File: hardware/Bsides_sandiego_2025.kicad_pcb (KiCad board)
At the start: 2 copper layers, 49.9 x 71.1 mm, 33 parts, among them J1 Conn_02x03_Odd_Even, J2 OLED, SW1 RESET, SW2 SW_SPDT, U1 CH32V003FxPx

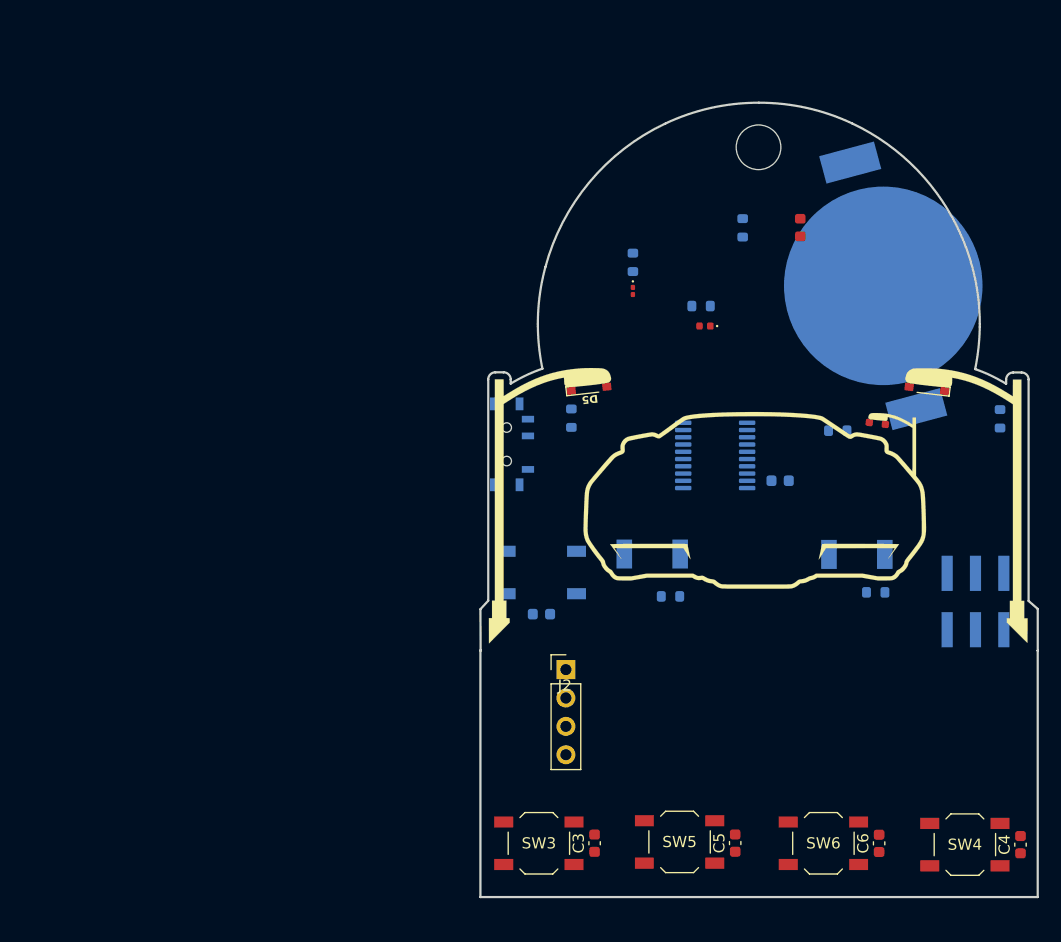
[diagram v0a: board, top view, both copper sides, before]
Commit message: feat(Hw):Update_Route
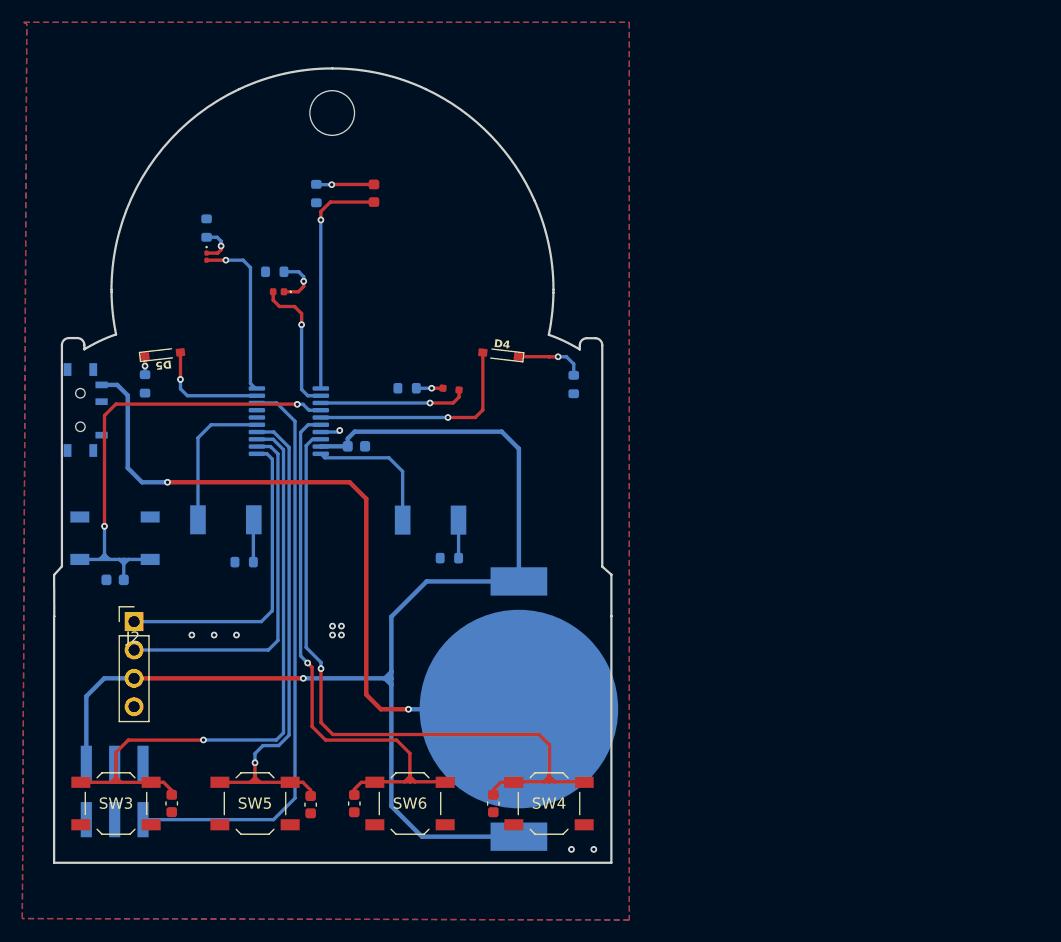
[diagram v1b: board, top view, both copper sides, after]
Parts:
- moved J1 78.9 mm to (67.1, 111.0)
- moved BT1 50.0 mm to (103.3, 103.6), turned to 90 degrees
- moved C4 47.4 mm to (101.0, 112.1)
- moved C6 47.1 mm to (88.5, 112.1)
- moved J2 38.9 mm to (68.8, 95.8)
- moved R8 38.8 mm to (93.3, 74.9)
- moved D1 38.3 mm to (75.3, 63.1)
- moved D3 38.3 mm to (90.3, 57.4)
- moved D7 38.3 mm to (95.4, 86.7)
- moved R1 38.3 mm to (75.3, 60.6)
- moved R2 38.3 mm to (81.4, 64.5)
- moved R7 38.3 mm to (97.1, 90.1)
- moved Ref** 38.3 mm to (86.6, 70.8)
- moved SW2 38.3 mm to (64.0, 76.8)
- moved U1 38.3 mm to (82.7, 77.8)
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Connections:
- C1 pad 2: VCC -> +3.3V
- J2 pad 3: VCC -> +3.3V
- U1 pad 1: /LED1 -> /LED3
- U1 pad 13: /LED8 -> /LEFT
- U1 pad 14: /LEFT -> /UP
- U1 pad 15: /UP -> /LED6
- U1 pad 19: /DOWN -> /LED5
- U1 pad 20: /RIGHT -> /LED1
- U1 pad 3: /LED3 -> /LED8
- U1 pad 6: /LED5 -> /DOWN
- U1 pad 8: /LED6 -> /RIGHT
- U1 pad 9: VCC -> +3.3V
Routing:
- net +3.3V: track 0.00 -> 109.1 mm, vias 0 -> 1
- net Net-(BT1--): track 0.00 -> 63.5 mm, vias 0 -> 2
- net /RIGHT: track 0.00 -> 62.0 mm, vias 0 -> 1
- net /LEFT: track 0.00 -> 56.7 mm, vias 0 -> 1
- net /SWDIO: track 0.00 -> 52.3 mm
- net /DOWN: track 0.00 -> 51.5 mm, vias 0 -> 1
- net /UP: track 0.00 -> 46.1 mm, vias 0 -> 1
- net /RST: track 0.00 -> 43.5 mm, vias 0 -> 2
- net /SCL: track 0.00 -> 32.1 mm
- net /SDA: track 0.00 -> 27.9 mm
- net /LED3: track 0.00 -> 21.0 mm, vias 0 -> 1
- net /LED4: track 0.00 -> 19.9 mm, vias 0 -> 1
- net /LED1: track 0.00 -> 15.3 mm, vias 0 -> 1
- net /LED8: track 0.00 -> 13.2 mm, vias 0 -> 1
- net /LED6: track 0.00 -> 13.1 mm
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- added copper zone on B.Cu, net GND
- added copper zone on F.Cu, net GND
